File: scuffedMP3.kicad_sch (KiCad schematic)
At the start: 12 parts, among them IC1 TTP229-BSF, J1 OLED, J2 Micro_SD_Card, J3 AudioJack3, J4 Conn_01x16_Pin, U1 ESP32-WROVER-E, U2 TP4056-42-ESOP8, U3 CP2102N-Axx-xQFN24, U4 MCP1825S, U5 PCM5102A

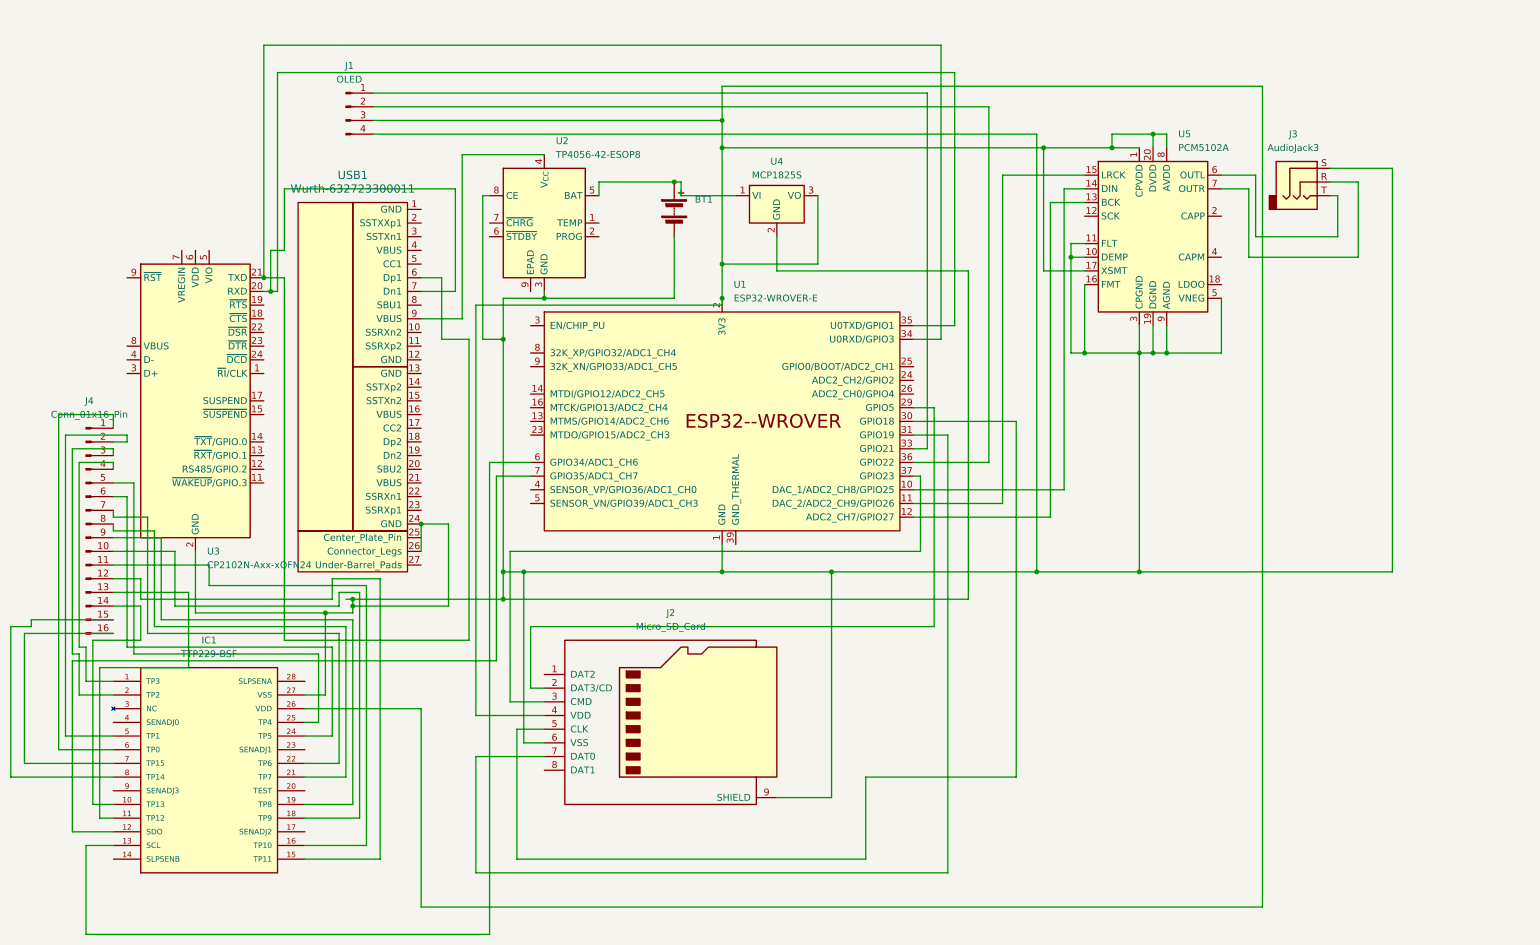
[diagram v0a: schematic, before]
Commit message: progress
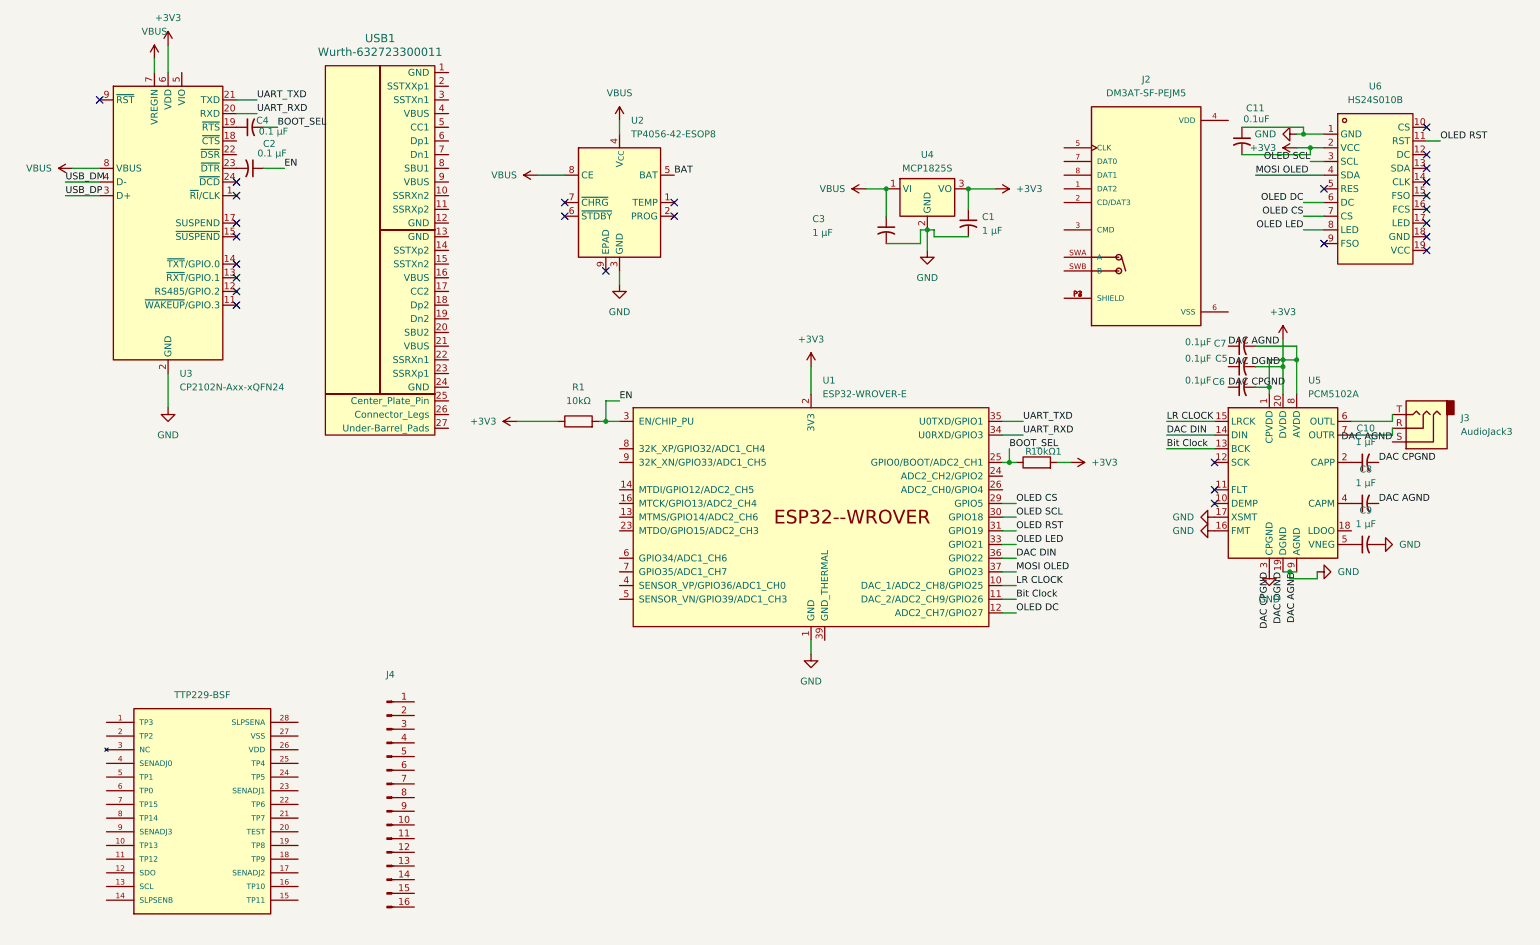
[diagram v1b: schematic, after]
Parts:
- removed BT1: Battery, Connector_JST:JST_PH_S2B-PH-K_1x02_P2.00mm_Horizontal, symbol Device:Battery
- removed J1: OLED, OLED:128x64OLED, symbol Connector:Conn_01x04_Pin
- removed J2: Micro_SD_Card, Connector_Card:SD_Card_Device_16mm_SlotDepth, symbol Connector:Micro_SD_Card
- added 10kΩ1: R, symbol Device:R
- added C1, C3: 1 µF, Capacitor_SMD:C_0603_1608Metric, symbol Device:C_Small_US
- added C10, C8, C9: 1 µF, symbol Device:C_Small_US
- added C11: 0.1uF, symbol Device:C_Small_US
- added C2, C4: 0.1 µF, symbol Device:C_Small_US
- added C5, C6, C7: 0.1µF, symbol Device:C_Small_US
- added J2: DM3AT-SF-PEJM5, DM3AT-SF-PEJM5:HRS_DM3AT-SF-PEJM5, symbol DM3AT-SF-PEJM5:DM3AT-SF-PEJM5
- added R1: 10kΩ, symbol Device:R
- added U6: HS24S010B, easyeda2kicad:LCD-TH_L72.3-W43.0_HS24S010B, symbol OLED:HS24S010B
- J4: footprint Library:ScrollWheel-40x12mm -> Wheel:ScrollWheel-40x20mm
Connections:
- net GND: now reaches J3.S, U1.1 (GND), U1.15 (GND), U1.38 (GND), U2.3 (GND), U3.2 (GND), U3.25 (GND), U4.2 (GND), U5.16 (FMT), U5.19 (DGND), U5.3 (CPGND), U5.9 (AGND)
- net GND: now also U5.17 (XSMT), C1.2, C10.2, C11.1, C3.2, C5.1, C6.1, C7.1, C8.2, C9.2, U6.1 (GND); no longer IC1.27 (VSS), U2.8 (CE), U5.10 (DEMP), U5.11 (FLT), U5.5 (VNEG), USB1.24 (GND), USB1.26 (Connector_Legs)
- net at USB1.9 (VBUS): no longer U2.4 (V_{CC})
- net at J4.1 (Pin_1): no longer IC1.6 (TP0)
- net at J4.10 (Pin_10): no longer IC1.18 (TP9)
- net at J4.11 (Pin_11): no longer IC1.16 (TP10)
- net at J4.12 (Pin_12): no longer IC1.15 (TP11)
- net at J4.13 (Pin_13): no longer IC1.11 (TP12)
- net at J4.14 (Pin_14): no longer IC1.10 (TP13)
- net at J4.15 (Pin_15): no longer IC1.8 (TP14)
- net at J4.16 (Pin_16): no longer IC1.7 (TP15)
- net at J4.2 (Pin_2): no longer IC1.5 (TP1)
- net at J4.3 (Pin_3): no longer IC1.2 (TP2)
- net at J4.4 (Pin_4): no longer IC1.1 (TP3)
- net at J4.5 (Pin_5): no longer IC1.25 (TP4)
- net at J4.6 (Pin_6): no longer IC1.24 (TP5)
- net at J4.7 (Pin_7): no longer IC1.22 (TP6)
- net at J4.8 (Pin_8): no longer IC1.21 (TP7)
- net at J4.9 (Pin_9): no longer IC1.19 (TP8)
- net DAC DIN: now reaches U5.14 (DIN)
- net DAC DIN: now also U1.36 (GPIO22); no longer U1.10 (DAC_1/ADC2_CH8/GPIO25)
- net Bit Clock: now reaches U1.11 (DAC_2/ADC2_CH9/GPIO26)
- net Bit Clock: now also U5.13 (BCK); no longer U5.15 (LRCK)
- net OLED DC: now reaches U1.12 (ADC2_CH7/GPIO27)
- net OLED DC: now also U6.6 (DC); no longer U5.13 (BCK)
- net +3V3: now reaches U1.2 (3V3), U4.3 (VO), U5.1 (CPVDD), U5.20 (DVDD), U5.8 (AVDD)
- net +3V3: now also U3.6 (VDD), 10kΩ1.2, C1.1, C11.2, C5.2, C6.2, C7.2, R1.1, U6.2 (VCC); no longer IC1.26 (VDD), U5.17 (XSMT)
- net BOOT_SEL: now reaches U1.25 (GPIO0/BOOT/ADC2_CH1)
- net BOOT_SEL: now also 10kΩ1.1, C4.2
- net OLED CS: now reaches U1.29 (GPIO5)
- net OLED CS: now also U6.7 (CS)
- net EN: now reaches U1.3 (EN/CHIP_PU)
- net EN: now also C2.1, R1.2
- net OLED SCL: now reaches U1.30 (GPIO18)
- net OLED SCL: now also U6.3 (SCL)
- net OLED RST: now reaches U1.31 (GPIO19)
- net OLED RST: now also U6.11 (RST)
- net OLED LED: now reaches U1.33 (GPIO21)
- net OLED LED: now also U6.8 (LED)
- net MOSI OLED: now reaches U1.37 (GPIO23)
- net MOSI OLED: now also U6.4 (SDA)
- net at U1.6 (GPIO34/ADC1_CH6): no longer IC1.13 (SCL)
- net at U1.7 (GPIO35/ADC1_CH7): no longer IC1.12 (SDO)
- net at U5.2 (CAPP): now also C10.1
- net at U5.4 (CAPM): now also C8.1
- net BAT: now reaches U2.5 (BAT)
- net BAT: no longer U4.1 (VI)
- net at U3.19 (~{RTS}): now also C4.1
- net at U3.23 (~{DTR}): now also C2.2
- net USB_DP: now reaches U3.3 (D+)
- net USB_DM: now reaches U3.4 (D-)
- net VBUS: now reaches U3.7 (VREGIN)
- net VBUS: now also U2.4 (V_{CC}), U2.8 (CE), U3.8 (VBUS), U4.1 (VI), C3.1
- new net: C9.1, U5.5 (VNEG)
- new net: J2.P1 (SHIELD), J2.P2 (SHIELD), J2.P3 (SHIELD), J2.P4 (SHIELD)
- new net LR CLOCK: U1.10 (DAC_1/ADC2_CH8/GPIO25), U5.15 (LRCK)
- new net UART_RXD: U1.34 (U0RXD/GPIO3), U3.20 (RXD)
- new net UART_TXD: U1.35 (U0TXD/GPIO1), U3.21 (TXD)
- now unconnected: USB1.6 (Dp1), USB1.7 (Dn1)
- no-connect marks 0 -> 28
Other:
- moved on the sheet: J3, J4, U1, U2, U3, U4, U5, USB1
